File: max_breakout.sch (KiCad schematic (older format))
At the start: 51 parts, among them J1 AVR-JTAG-10, J2 Conn_01x19, J3 USB_B_Micro, J4 Conn_01x19, Q1 IRLML6402, SW1 SW_DIP_x06, U1 74HCT365, U2 CPLD - EPM7032STC44, U3 74HCT2G125, U4 MAX40200AUK, U5 MAX40200AUK, U6 74AHCT1G04, U7 74AHCT1G04, X1 CTX-636 50mhz

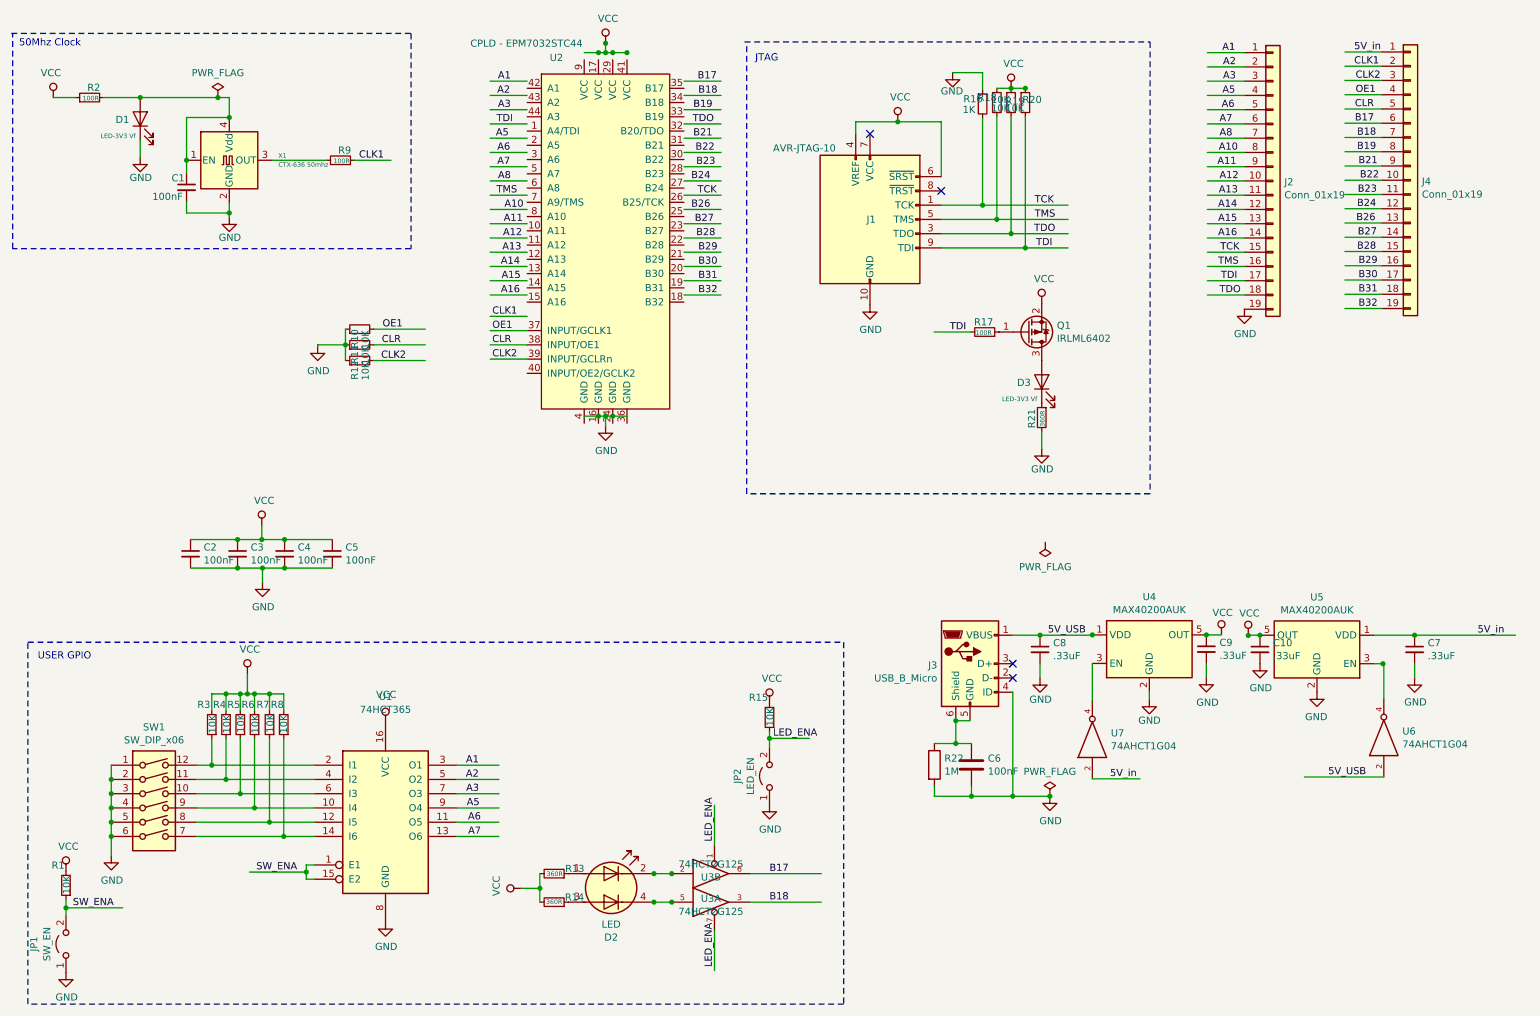
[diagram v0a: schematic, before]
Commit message: start routing
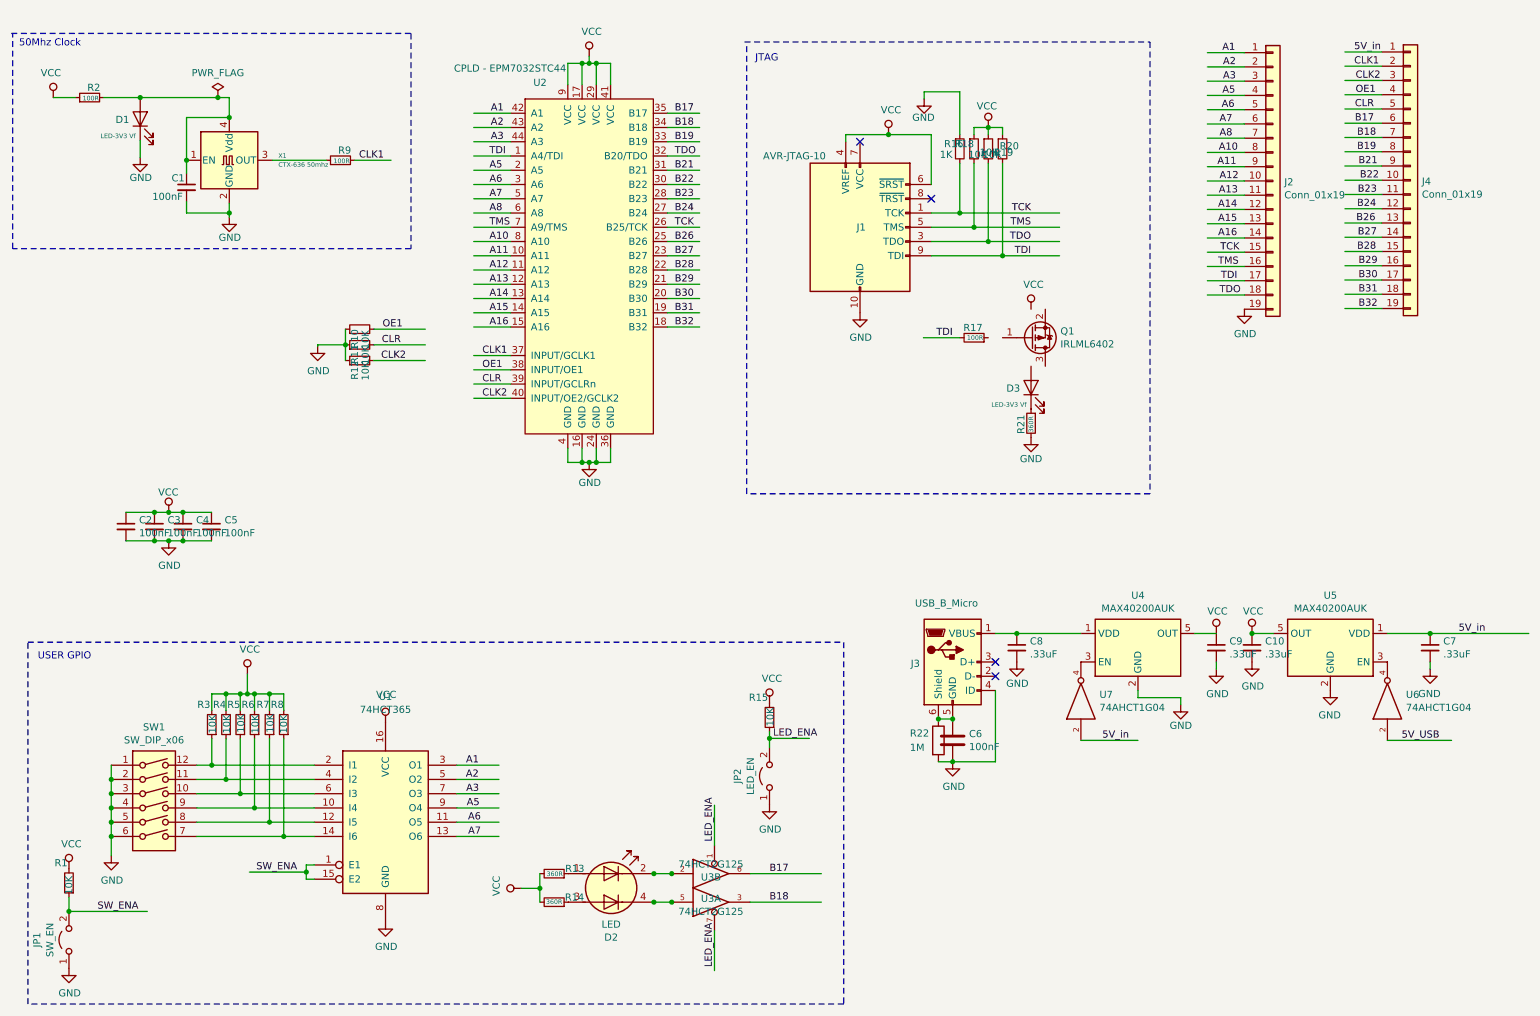
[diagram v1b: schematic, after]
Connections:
- wire segments 234 -> 226
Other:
- moved on the sheet: C10, C2, C3, C4, C5, C6, C7, C8, D3, J1, J3, JP1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

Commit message: version 1.0
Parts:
- removed U6, U7: 74AHCT1G04, Package_TO_SOT_SMD:SOT-23-5_HandSoldering, symbol 74xGxx:74AHCT1G04
- added C2, C7: 100nF, Capacitor_SMD:C_0603_1608Metric_Pad1.05x0.95mm_HandSolder, symbol max_breakout-rescue:C_Small-Device
- D1: value LED-3V3 Vf -> Blue 3V3 Vf
- D2: renamed from D3; value LED-3V3 Vf -> Green
- J1: renamed from J4; value Conn_01x19 -> Right
- J2: value Conn_01x19 -> Left
- Q1: symbol Transistor_FET:IRLML6402 -> max_breakout-rescue:IRLML6402-Transistor_FET
- R10: renamed from R12; value 10K -> 1K
- R7: renamed from R10; value 10K -> 1K
- R9: renamed from R11; value 10K -> 1K
- U1: renamed from U2; value CPLD - EPM7032STC44 -> EPM7032STC44
- U2: renamed from U4; symbol Analog_Switch:MAX40200AUK -> max_breakout-rescue:MAX40200AUK-Analog_Switch
- U3: renamed from U5; symbol Analog_Switch:MAX40200AUK -> max_breakout-rescue:MAX40200AUK-Analog_Switch
- renumbered C7 to C10, C10 to C11, C6 to C12, C2 to C3, C3 to C4, C4 to C5, C5 to C6, D2 to D3, J1 to J3, J3 to J4, JP2 to JP1, JP1 to JP2, R2 to R1, R21 to R11, R3 to R12, R4 to R13, R5 to R14, R6 to R15, R7 to R16, R8 to R17, R15 to R18, R22 to R19, R16 to R2, R13 to R20, R1 to R21, R14 to R22, R18 to R3, R19 to R4, R20 to R5, R9 to R6, R17 to R8, U1 to U4, U3 to U5
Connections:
- net labels removed: 5V_USB
- wire segments 226 -> 231
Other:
- note added: "Note: LED must have a forward voltage of 3V3"
- moved on the sheet: C1, C10, C11, C12, C3, C4, C5, C6, C8, C9, D2, J4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
